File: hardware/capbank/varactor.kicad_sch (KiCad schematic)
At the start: 12 parts, among them U2 OPA2202IDR

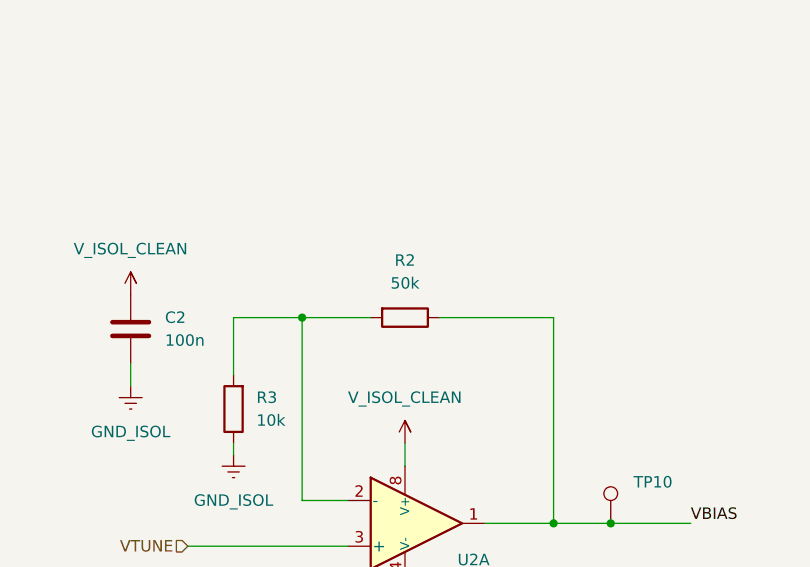
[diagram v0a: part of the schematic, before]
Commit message: KiCad changes
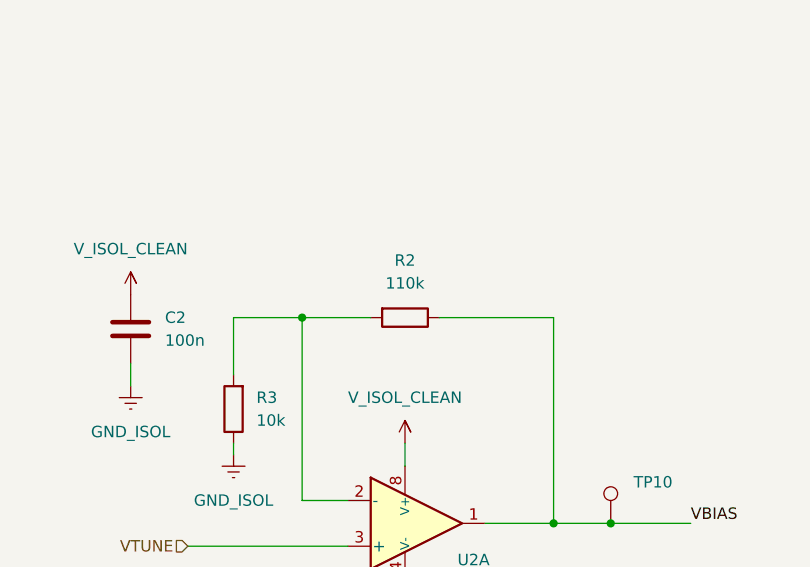
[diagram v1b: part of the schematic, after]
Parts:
- R2: value 50k -> 110k
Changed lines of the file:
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@@
 			)
 		)
-		(property "Value" "50k"
+		(property "Value" "110k"
 			(at 81.28 66.04 90)
 			(effects
